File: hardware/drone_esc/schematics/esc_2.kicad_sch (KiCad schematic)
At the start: 32 parts, among them Q10 BSC016N04LS, Q11 BSC016N04LS, Q12 BSC016N04LS, Q7 BSC016N04LS, Q8 BSC016N04LS, Q9 BSC016N04LS, U6 FD6288Q

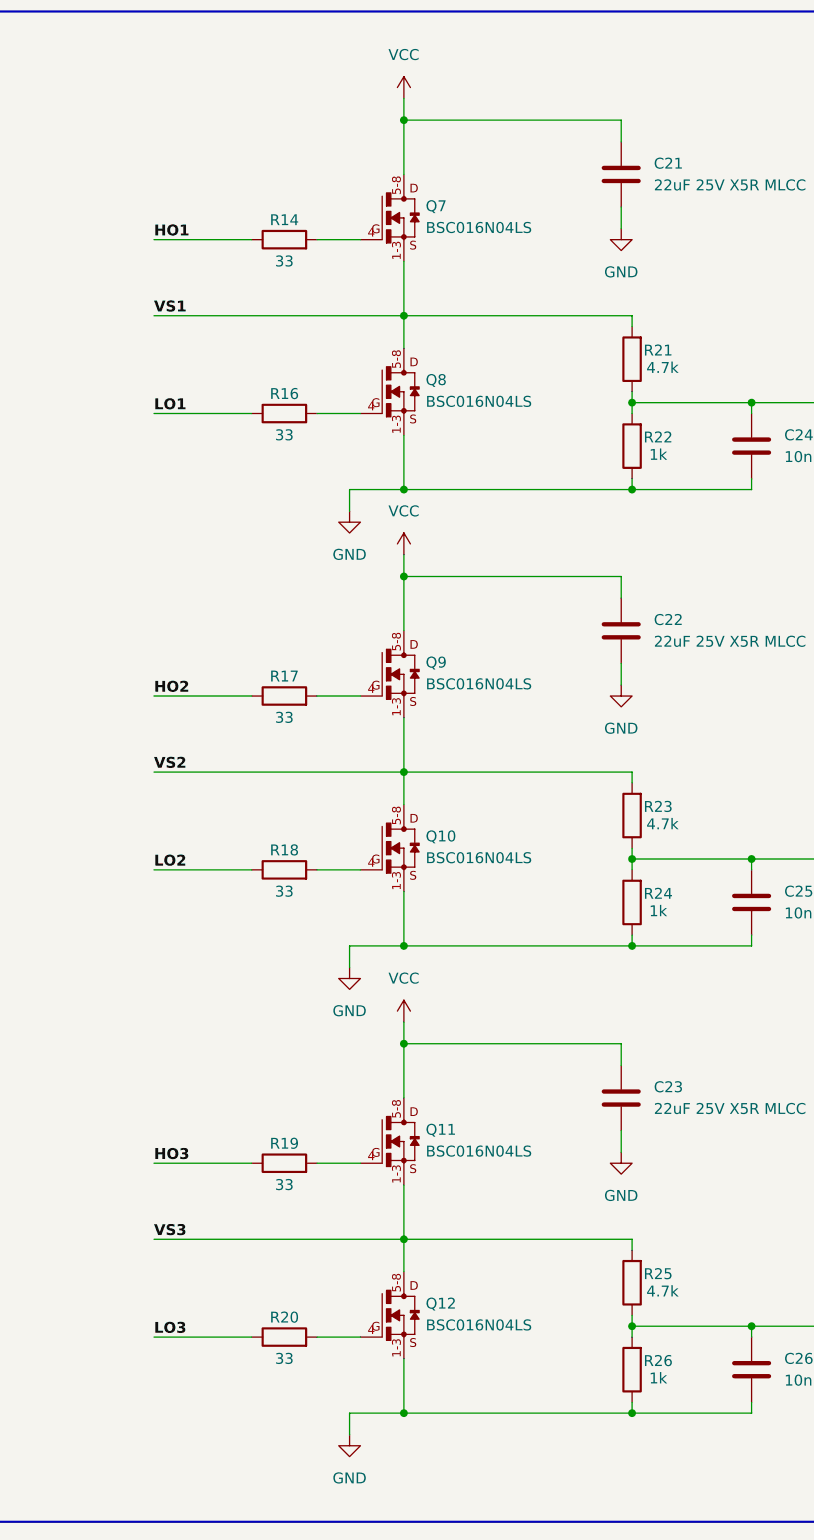
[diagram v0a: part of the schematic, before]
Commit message: replaced some of the schematics
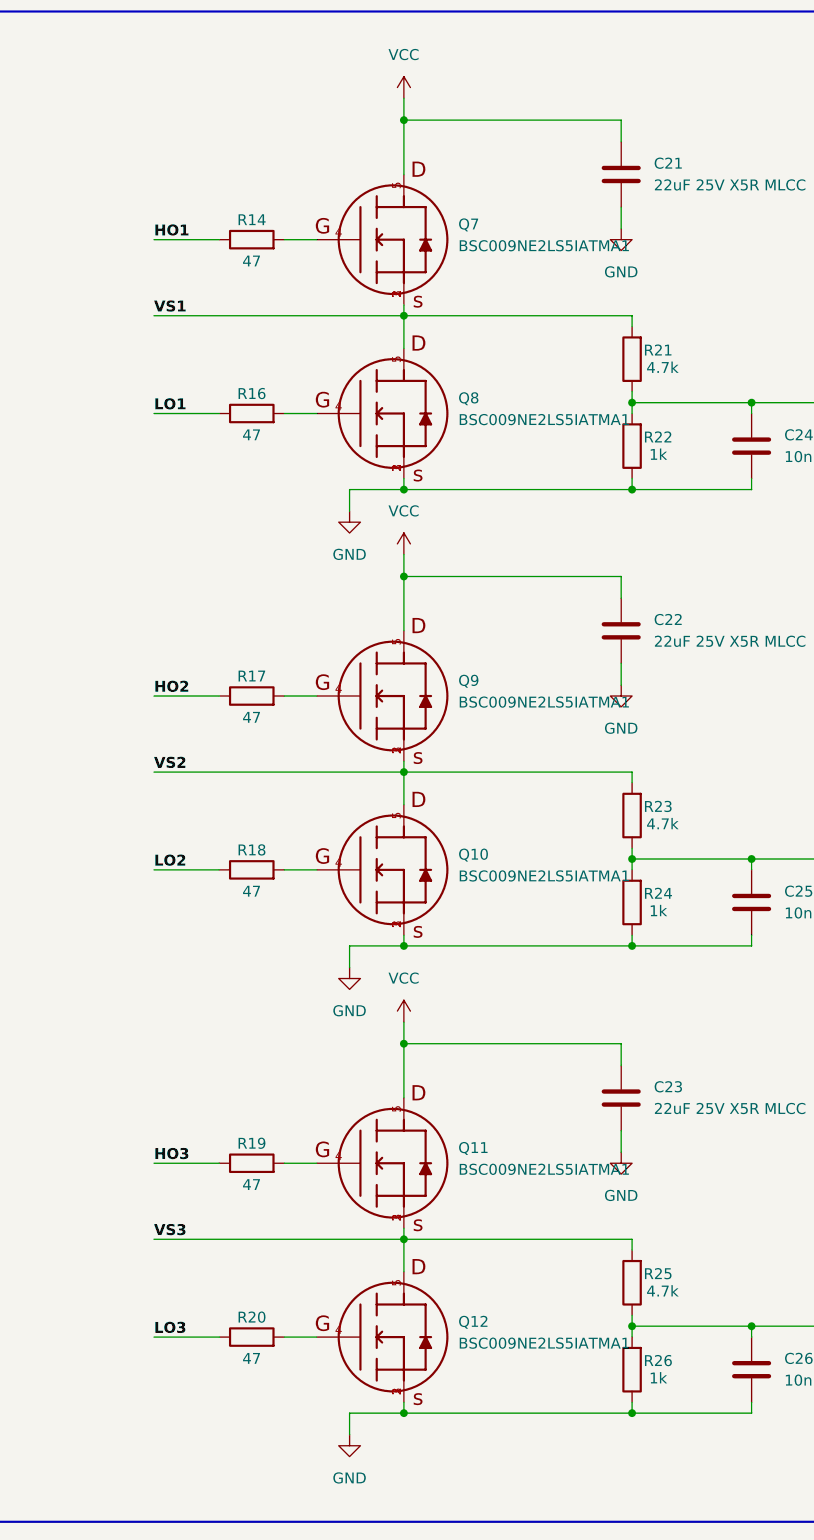
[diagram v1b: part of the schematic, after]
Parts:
- removed Q10, Q11, Q12, Q7, Q8, Q9: BSC016N04LS, Drone_components:BSC016N04LS, symbol Drone_components:BSC016N04LS
- added Q10, Q11, Q12, Q7, Q8, Q9: BSC009NE2LS5IATMA1, Drone_components:BSC093N04LSGATMA1, symbol Drone_components:BSC009NE2LS5IATMA1
- C21, C22, C23: footprint Capacitor_SMD:C_1210_3225Metric -> Capacitor_SMD:C_0805_2012Metric; JLCPCB part C12891 -> C45783
- R14, R16, R17, R18, R19, R20: value 33 -> 47
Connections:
- net GND: now also Q10.1, Q10.2, Q10.3, Q12.1, Q12.2, Q12.3, Q8.1, Q8.2, Q8.3
- net VCC: now also Q11.5, Q7.5, Q9.5
- net VS1: now also Q7.1, Q7.2, Q7.3, Q8.5
- net VS2: now also Q10.5, Q9.1, Q9.2, Q9.3
- net VS3: now also Q11.1, Q11.2, Q11.3, Q12.5
- net at R19.2: now also Q11.4
- net at R17.2: now also Q9.4
- net at R18.2: now also Q10.4
- net at R14.2: now also Q7.4
- net at R16.2: now also Q8.4
- net at R20.2: now also Q12.4
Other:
- moved on the sheet: R14, R16, R17, R18, R19, R20
